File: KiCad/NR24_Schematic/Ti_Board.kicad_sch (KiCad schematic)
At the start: 2 parts, among them J5 Dash TI Connection, J8 CAN Connector

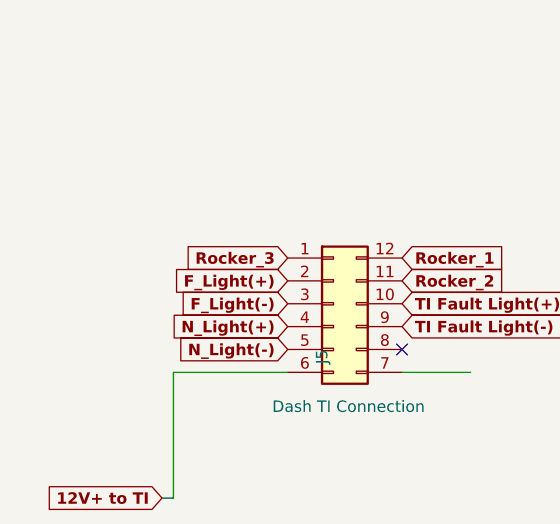
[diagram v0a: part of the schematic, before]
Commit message: B-? where are stops connected to
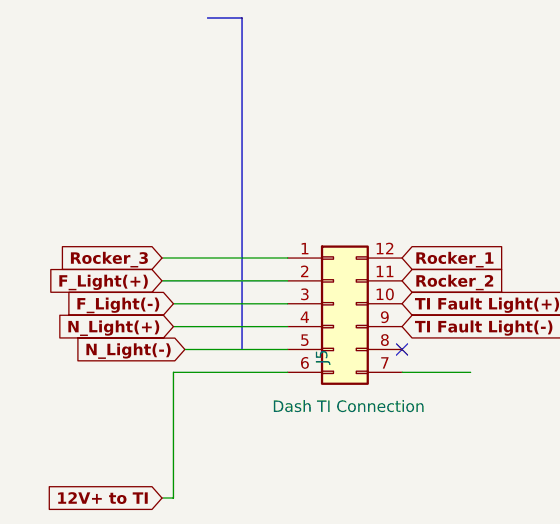
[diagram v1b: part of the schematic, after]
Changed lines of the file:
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@@
   (no_connect (at 186.69 82.55))
   (no_connect (at 116.84 82.55))
+  (wire (pts (xy 90.17 74.93) (xy 104.14 74.93))
+    (stroke (width 0) (type default))
+  )
+  (bus (pts (xy 99.06 82.55) (xy 99.06 45.72))
+    (stroke (width 0) (type default))
+  )
   (wire (pts (xy 91.44 85.09) (xy 104.14 85.09))
+    (stroke (width 0) (type default))
+  )
+  (wire (pts (xy 91.44 80.01) (xy 104.14 80.01))
+    (stroke (width 0) (type default))
+  )
+  (wire (pts (xy 91.44 77.47) (xy 104.14 77.47))
+    (stroke (width 0) (type default))
+  )
+  (bus (pts (xy 95.25 45.72) (xy 99.06 45.72))
+    (stroke (width 0) (type default))
+  )
+  (wire (pts (xy 90.17 72.39) (xy 104.14 72.39))
+    (stroke (width 0) (type default))
+  )
+  (wire (pts (xy 92.71 82.55) (xy 104.14 82.55))
     (stroke (width 0) (type default))
   )
@@
     (stroke (width 0) (type default))
   )
-  (global_label "F_Light(-)" (shape input) (at 104.14 77.47 180) (fields_autoplaced)
+  (global_label "F_Light(-)" (shape input) (at 91.44 77.47 180) (fields_autoplaced)
     (effects (font (size 1.27 1.27) (thickness 0.254) bold) (justify right))
-    (property "Intersheetrefs" "${INTERSHEET_REFS}" (at 90.7002 77.47 0)
+    (property "Intersheetrefs" "${INTERSHEET_REFS}" (at 78.0002 77.47 0)
       (effects (font (size 1.27 1.27) (thickness 0.254) bold) (justify right) hide)
     )
   )
-  (global_label "F_Light(+)" (shape input) (at 104.14 74.93 180) (fields_autoplaced)
+  (global_label "F_Light(+)" (shape input) (at 90.17 74.93 180) (fields_autoplaced)
     (effects (font (size 1.27 1.27) (thickness 0.254) bold) (justify right))
-    (property "Intersheetrefs" "${INTERSHEET_REFS}" (at 90.7002 74.93 0)
+    (property "Intersheetrefs" "${INTERSHEET_REFS}" (at 76.7302 74.93 0)
       (effects (font (size 1.27 1.27) (thickness 0.254) bold) (justify right) hide)
     )
@@
     )
   )
-  (global_label "N_Light(-)" (shape input) (at 104.14 82.55 180) (fields_autoplaced)
+  (global_label "N_Light(-)" (shape input) (at 92.71 82.55 180) (fields_autoplaced)
     (effects (font (size 1.27 1.27) (thickness 0.254) bold) (justify right))
-    (property "Intersheetrefs" "${INTERSHEET_REFS}" (at 90.4583 82.55 0)
+    (property "Intersheetrefs" "${INTERSHEET_REFS}" (at 79.0283 82.55 0)
       (effects (font (size 1.27 1.27) (thickness 0.254) bold) (justify right) hide)
     )
@@
     )
   )
-  (global_label "Rocker_3" (shape input) (at 104.14 72.39 180) (fields_autoplaced)
+  (global_label "Rocker_3" (shape input) (at 90.17 72.39 180) (fields_autoplaced)
     (effects (font (size 1.27 1.27) (thickness 0.254) bold) (justify right))
-    (property "Intersheetrefs" "${INTERSHEET_REFS}" (at 92.0912 72.39 0)
+    (property "Intersheetrefs" "${INTERSHEET_REFS}" (at 78.1212 72.39 0)
       (effects (font (size 1.27 1.27) (thickness 0.254) bold) (justify right) hide)
     )
@@
     )
   )
-  (global_label "N_Light(+)" (shape input) (at 104.14 80.01 180) (fields_autoplaced)
+  (global_label "N_Light(+)" (shape input) (at 91.44 80.01 180) (fields_autoplaced)
     (effects (font (size 1.27 1.27) (thickness 0.254) bold) (justify right))
-    (property "Intersheetrefs" "${INTERSHEET_REFS}" (at 90.4583 80.01 0)
+    (property "Intersheetrefs" "${INTERSHEET_REFS}" (at 77.7583 80.01 0)
       (effects (font (size 1.27 1.27) (thickness 0.254) bold) (justify right) hide)
     )
